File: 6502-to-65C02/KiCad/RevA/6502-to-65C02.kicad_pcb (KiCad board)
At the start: 2 copper layers, 54 x 23 mm, 6 parts

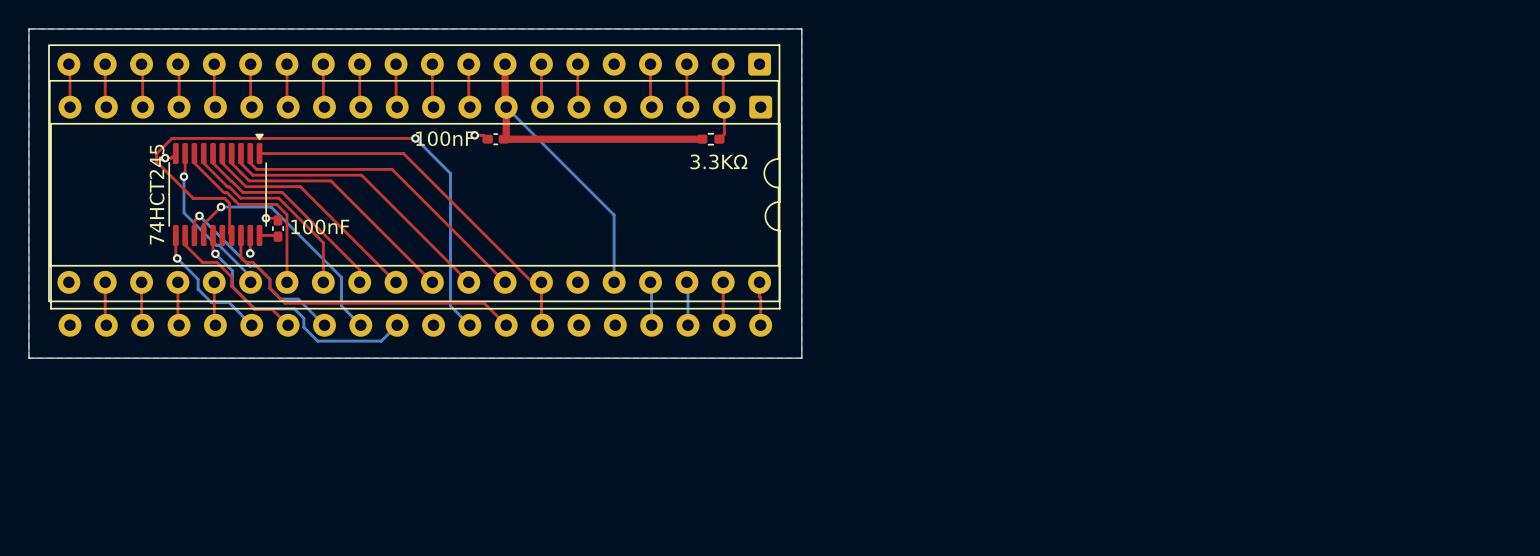
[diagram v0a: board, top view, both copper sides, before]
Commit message: Finalised design for testing
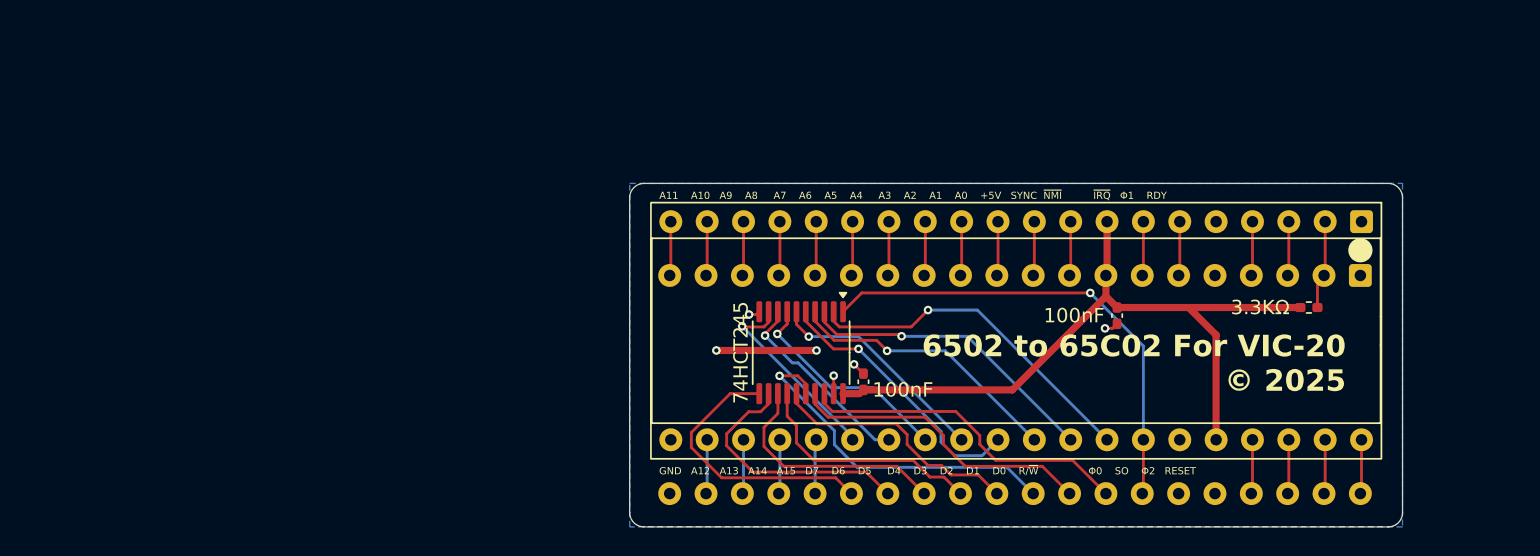
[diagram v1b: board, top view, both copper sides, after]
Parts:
- moved C1 58.9 mm to (146.0, 71.6), turned to -90 degrees
- moved UE10 43.5 mm to (163.0, 68.8)
- moved UE101 43.5 mm to (163.1, 65.0)
- moved R1 43.4 mm to (159.4, 71.0)
- moved UE102 42.2 mm to (123.9, 74.2)
- moved C2 30.8 mm to (128.3, 76.2), turned to 90 degrees
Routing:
- net /D2: track 0.00 -> 24.5 mm, vias 0 -> 1
- net /D1: track 42.3 -> 21.5 mm, vias 1 -> 0
- net +5V: track 36.0 -> 50.4 mm
- net /D7: track 9.19 -> 19.4 mm, vias 1 -> 0
- net /D6: track 10.6 -> 18.0 mm
- net GND: track 4.05 -> 10.9 mm, vias 4 -> 6
- net R/W: track 26.7 -> 33.4 mm, vias 0 -> 1
- net /D5: track 13.8 -> 16.6 mm, vias 1 -> 0
- net Net-(UE101-D7): track 11.1 -> 13.9 mm
- net Net-(UE101-D3): track 16.3 -> 18.9 mm, vias 0 -> 1
- net Net-(UE101-D0): track 21.9 -> 24.2 mm, vias 0 -> 1
- net Net-(UE101-D1): track 20.0 -> 21.3 mm, vias 0 -> 1
- net Net-(UE101-D2): track 18.2 -> 19.4 mm, vias 0 -> 1
- net Net-(UE101-D5): track 14.1 -> 15.2 mm, vias 0 -> 1
- net /D0: track 22.4 -> 23.3 mm
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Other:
- board size 54 x 23 mm -> 54 x 24 mm
- board text added: "6502 to 65C02 For VIC-20 © 2025"
- board text added: "A11 A10 A9 A8 A7 A6 A5 A4 A3 A2 A1 A0 +5V SYNC ~{NMI} ~{IRQ} Φ1 RDY"
- board text added: "Brett Hallen, Apr 2025 Port Macquarie, Australia www.youtube.com/@Brfff"
- board text added: "GND A12 A13 A14 A15 D7 D6 D5 D4 D3 D2 D1 D0 R/~{W} Φ0 SO Φ2 RESET"
